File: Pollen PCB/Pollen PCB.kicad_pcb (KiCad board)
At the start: 2 copper layers, 80 x 84 mm, 19 parts, among them J1 GY-GPS6MV2, J2 Adafruit Charge Controller, J3 Solar_panel, J4 Solar_panel, J5 Solar_charger, J6 Raspberry Pi, J7 Battery, Q1 Si2319CDS, Q2 MMBT2222A, Q3 MMBT2222A, Q4 Si2319CDS, U1 NB-IOT-BC660, U2 Pico, U3 XL6009_DC-DC, U4 DHT22, U5 INA219AxD, U6 INA219AxD, U7 DHT22

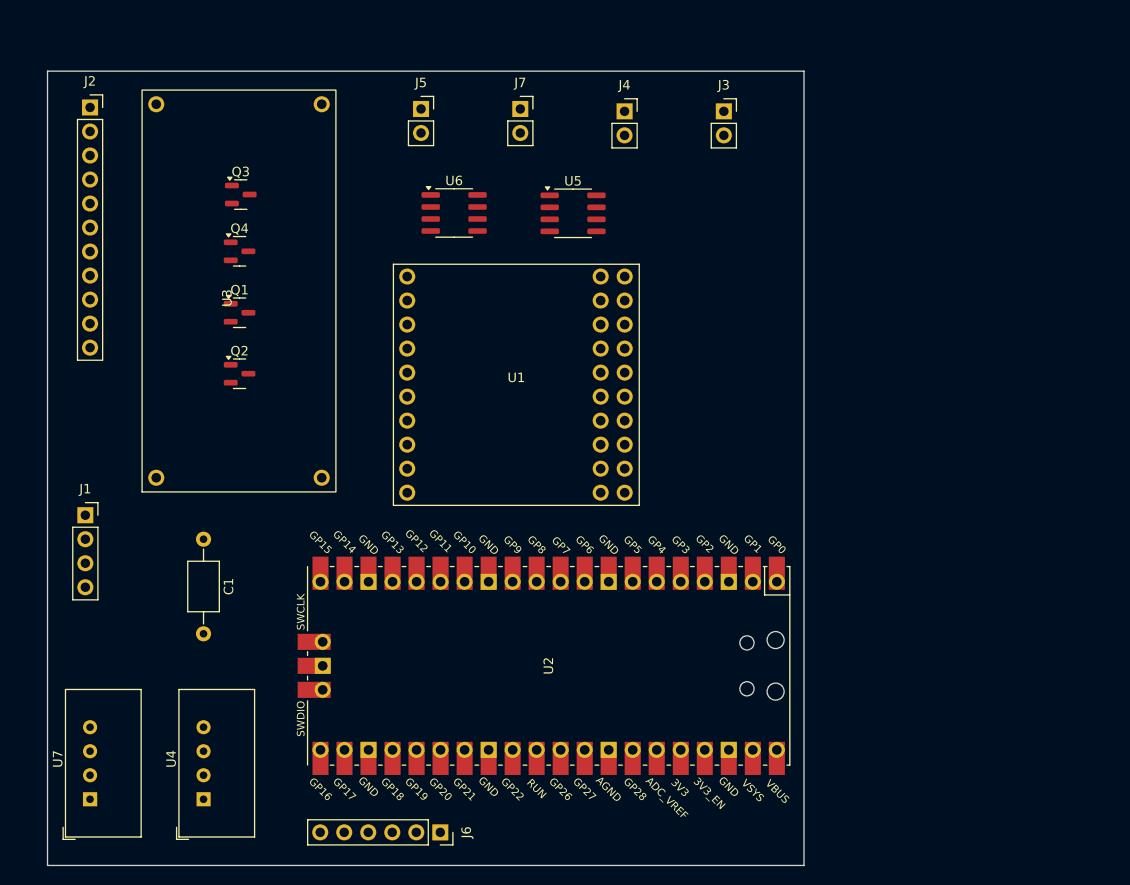
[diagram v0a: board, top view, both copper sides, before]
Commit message: Update PCB
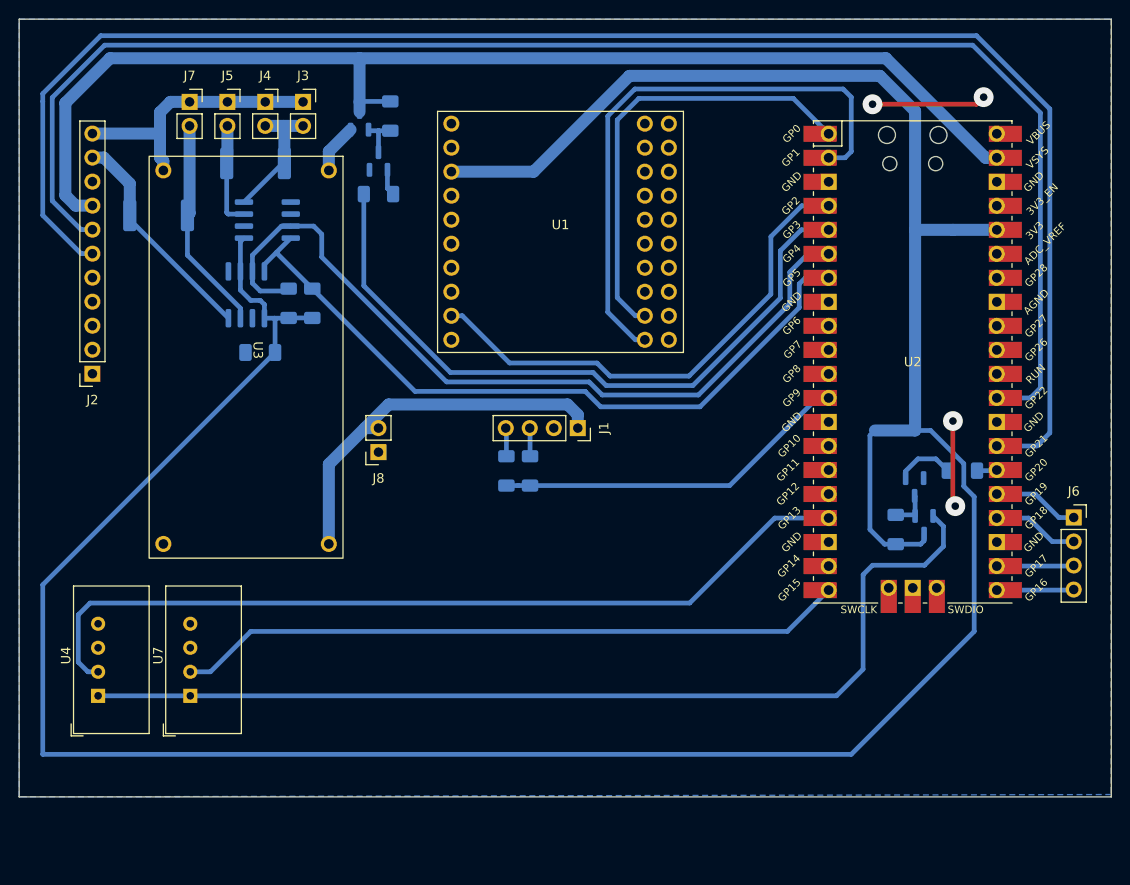
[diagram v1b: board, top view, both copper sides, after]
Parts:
- added J8: RPi power, Connector_PinSocket_2.54mm:PinSocket_1x02_P2.54mm_Vertical, F.Cu at (149.0, 100.3)
- added R1: 100m, Resistor_SMD:R_2512_6332Metric_Pad1.40x3.35mm_HandSolder, B.Cu at (136.0, 69.8)
- added R10: 10k, Resistor_SMD:R_1206_3216Metric_Pad1.30x1.75mm_HandSolder, B.Cu at (162.5, 102.3)
- added R2: 100m, Resistor_SMD:R_2512_6332Metric_Pad1.40x3.35mm_HandSolder, B.Cu at (125.8, 75.2)
- added R3: 10k, Resistor_SMD:R_1206_3216Metric_Pad1.30x1.75mm_HandSolder, B.Cu at (139.5, 84.5)
- added R4: 10k, Resistor_SMD:R_1206_3216Metric_Pad1.30x1.75mm_HandSolder, B.Cu at (142.0, 84.5)
- added R5: 10k, Resistor_SMD:R_1206_3216Metric_Pad1.30x1.75mm_HandSolder, B.Cu at (150.2, 64.8)
- added R6: 1k, Resistor_SMD:R_1206_3216Metric_Pad1.30x1.75mm_HandSolder, B.Cu at (149.0, 73.0)
- added R7: 1k, Resistor_SMD:R_1206_3216Metric_Pad1.30x1.75mm_HandSolder, B.Cu at (210.8, 102.2)
- added R8: 10k, Resistor_SMD:R_1206_3216Metric_Pad1.30x1.75mm_HandSolder, B.Cu at (203.7, 108.5)
- added R9: 5k1, Resistor_SMD:R_1206_3216Metric_Pad1.30x1.75mm_HandSolder, B.Cu at (165.0, 102.3)
- C1: footprint Capacitor_THT:C_Axial_L5.1mm_D3.1mm_P10.00mm_Horizontal -> Capacitor_SMD:C_1206_3216Metric_Pad1.33x1.80mm_HandSolder; moved to B.Cu
- J6: footprint Connector_PinSocket_2.54mm:PinSocket_1x06_P2.54mm_Vertical -> Connector_PinSocket_2.54mm:PinSocket_1x04_P2.54mm_Vertical
- Q1, Q2, Q3, Q4, U5, U6: moved to B.Cu
- moved Q4 78.0 mm to (206.7, 108.0), turned to -90 degrees
- moved Q3 77.7 mm to (205.7, 104.0), turned to -90 degrees
- moved J6 74.8 mm to (222.5, 107.2), turned to 0 degrees
- moved J1 52.9 mm to (170.1, 97.8), turned to -90 degrees
- moved U2 50.2 mm to (205.5, 90.8), turned to 0 degrees
- moved J3 44.5 mm to (141.0, 63.2)
- moved J4 38.0 mm to (137.0, 63.2)
- moved J7 35.0 mm to (129.0, 63.2)
- moved U5 32.3 mm to (137.2, 75.8), turned to 180 degrees
- moved J2 28.2 mm to (118.8, 92.0), turned to 180 degrees
- moved Q2 26.9 mm to (149.0, 69.5), turned to 90 degrees
- moved Q1 23.9 mm to (147.0, 65.2), turned to 90 degrees
- moved U6 23.6 mm to (135.0, 83.7), turned to -90 degrees
- moved C1 20.6 mm to (136.5, 89.8), turned to 180 degrees
- moved J5 20.5 mm to (133.0, 63.2)
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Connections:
- J1 pad 2: /GPS_RX -> unconnected-(J1-RX-Pad2)
- J1 pad 3: /GPS_TX -> Net-(J1-TX)
- J3 pad 1: /SOLAR_V+ -> GND
- J3 pad 2: GND -> /SOLAR_V+
- J4 pad 1: /SOLAR_V+ -> GND
- J4 pad 2: GND -> /SOLAR_V+
- J5 pad 1: /CHARGER_V+ -> GND
- J5 pad 2: GND -> /CHARGER_V+
- J6 pad 1: +5V -> /RPI_MOSI
- J6 pad 2: GND -> /RPI_SCK
- J6 pad 3: /RPI_MOSI -> /RPI_CS
- J6 pad 4: /RPI_SCK -> /RPI_MISO
- J7 pad 1: /BATTERY+ -> GND
- J7 pad 2: GND -> /BATTERY+
- U2 pad 11: /GPS_RX -> unconnected-(U2-GPIO8-Pad11)
- U2 pad 14: /CHARGER_CHG -> unconnected-(U2-GPIO10-Pad14)
- U2 pad 15: /CHARGER_PGOOD -> unconnected-(U2-GPIO11-Pad15)
- U2 pad 17: unconnected-(U2-GPIO13-Pad17) -> /DHT_1
- U2 pad 19: /DHT_1 -> unconnected-(U2-GPIO14-Pad19)
- U2 pad 26: unconnected-(U2-GPIO20-Pad26) -> /3V3_SENSOR_CONTROL
- U2 pad 27: unconnected-(U2-GPIO21-Pad27) -> /CHARGER_PGOOD
- U2 pad 29: unconnected-(U2-GPIO22-Pad29) -> /CHARGER_CHG
- U2 pad 4: /3V3_SENSOR_CONTROL -> /NB-IOT_RST
- U2 pad 9: /NB-IOT_RST -> unconnected-(U2-GPIO6-Pad9)
- U6 pad 7: /CHARGER_LIPO -> /BATTERY+
- U6 pad 8: /BATTERY+ -> /CHARGER_LIPO
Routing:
- net +3V3: track 0.00 -> 319.7 mm
- net /CHARGER_PGOOD: track 0.00 -> 172.5 mm
- net /CHARGER_CHG: track 0.00 -> 160.3 mm
- net +BATT: track 0.00 -> 126.9 mm
- net +3V3_SENSOR: track 0.00 -> 105.5 mm
- net /DHT_1: track 0.00 -> 91.1 mm
- net /SDA: track 0.00 -> 86.4 mm
- net /SCL: track 0.00 -> 77.0 mm
- net /5V_CONTROL: track 0.00 -> 73.0 mm
- net /DHT_2: track 0.00 -> 71.1 mm
- net /NB-IOT_TX: track 0.00 -> 61.6 mm
- net /NB-IOT_RST: track 0.00 -> 53.6 mm
- net GND: track 0.00 -> 53.3 mm, vias 0 -> 4
- net /NB-IOT_RX: track 0.00 -> 47.4 mm
- net +5V: track 0.00 -> 40.7 mm
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- added copper zone on B.Cu, net GND
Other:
- board size 80 x 84 mm -> 115.5 x 82.2 mm
